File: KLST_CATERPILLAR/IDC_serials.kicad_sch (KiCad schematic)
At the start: 0 parts

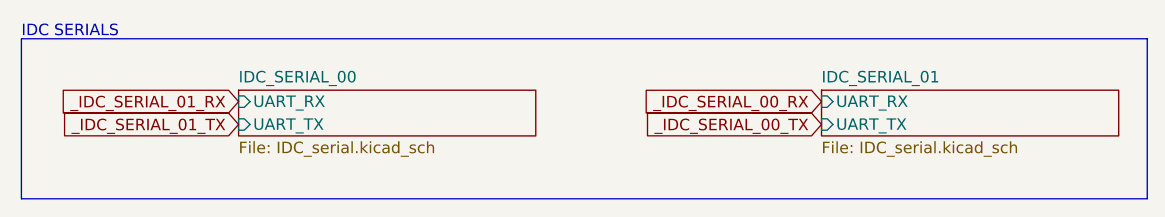
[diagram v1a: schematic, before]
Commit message: reduced modules
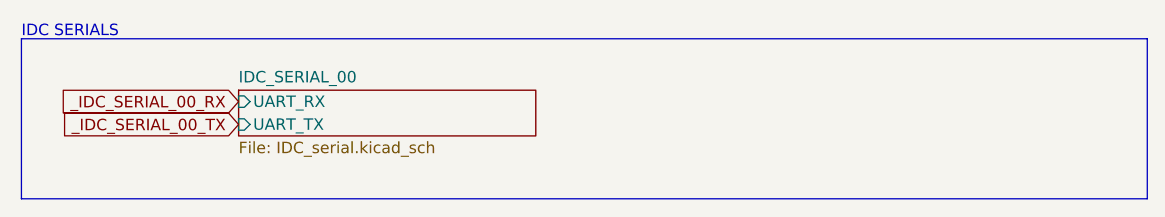
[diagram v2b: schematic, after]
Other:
- removed sheet IDC_SERIAL_01
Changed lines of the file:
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@@
 	(global_label "_IDC_SERIAL_00_TX"
-		(shape input)
-		(at 104.14 24.765 180)
-		(fields_autoplaced yes)
-		(effects
-			(font
-				(size 1.27 1.27)
-			)
-			(justify right)
-		)
-		(property "Intersheetrefs" "${INTERSHEET_REFS}"
-			(at 83.2729 24.765 0)
-			(effects
-				(font
-					(size 1.27 1.27)
-				)
-				(justify right)
-				(hide yes)
-			)
-		)
-	)
-	(global_label "_IDC_SERIAL_01_TX"
 		(shape input)
 		(at 39.37 24.765 180)
@@
 		)
 		(property "Intersheetrefs" "${INTERSHEET_REFS}"
-			(at 18.5029 24.765 0)
+			(at 18.4235 24.765 0)
 			(effects
 				(font
@@
 	(global_label "_IDC_SERIAL_00_RX"
 		(shape input)
-		(at 104.14 22.225 180)
-		(fields_autoplaced yes)
-		(effects
-			(font
-				(size 1.27 1.27)
-			)
-			(justify right)
-		)
-		(property "Intersheetrefs" "${INTERSHEET_REFS}"
-			(at 82.9705 22.225 0)
-			(effects
-				(font
-					(size 1.27 1.27)
-				)
-				(justify right)
-				(hide yes)
-			)
-		)
-	)
-	(global_label "_IDC_SERIAL_01_RX"
-		(shape input)
 		(at 39.37 22.225 180)
 		(fields_autoplaced yes)
@@
 		)
 		(property "Intersheetrefs" "${INTERSHEET_REFS}"
-			(at 18.2005 22.225 0)
+			(at 18.1211 22.225 0)
 			(effects
 				(font
@@
 				)
 			)
-		)
-	)
-	(sheet
-		(at 104.14 20.955)
-		(size 33.02 5.08)
-		(fields_autoplaced yes)
-		(stroke
-			(width 0.1524)
-			(type solid)
-		)
-		(fill
-			(color 0 0 0 0.0000)
-		)
-		(property "Sheetname" "IDC_SERIAL_01"
-			(at 104.14 20.2434 0)
-			(effects
-				(font
-					(size 1.27 1.27)
-				)
-				(justify left bottom)
-			)
-		)
-		(property "Sheetfile" "IDC_serial.kicad_sch"
-			(at 104.14 26.6196 0)
-			(effects
-				(font
-					(size 1.27 1.27)
-				)
-				(justify left top)
-			)
-		)
-		(pin "UART_RX" input
-			(at 104.14 22.225 180)
-			(effects
-				(font
-					(size 1.27 1.27)
-				)
-				(justify left)
-			)
-		)
-		(pin "UART_TX" input
-			(at 104.14 24.765 180)
-			(effects
-				(font
-					(size 1.27 1.27)
-				)
-				(justify left)
-			)
-		)
-		(instances
-			(project "KLST_CATERPILLAR"
-				(path "/b4513875-4c57-4720-bcc5-43ead67fe18f/8093d0e6-fdc1-46b4-b622-445b9f3a15e0"
-					(page "12")
-				)
-			)
